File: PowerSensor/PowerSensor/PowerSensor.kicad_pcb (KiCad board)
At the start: 2 copper layers, 40.8 x 26.4 mm, 13 parts, among them J1 Screw_Terminal_01x02, J2 Screw_Terminal_01x05, J3 Screw_Terminal_01x02, J4 Screw_Terminal_01x02, U1 ACS712ELCTR-20A-T_NRND

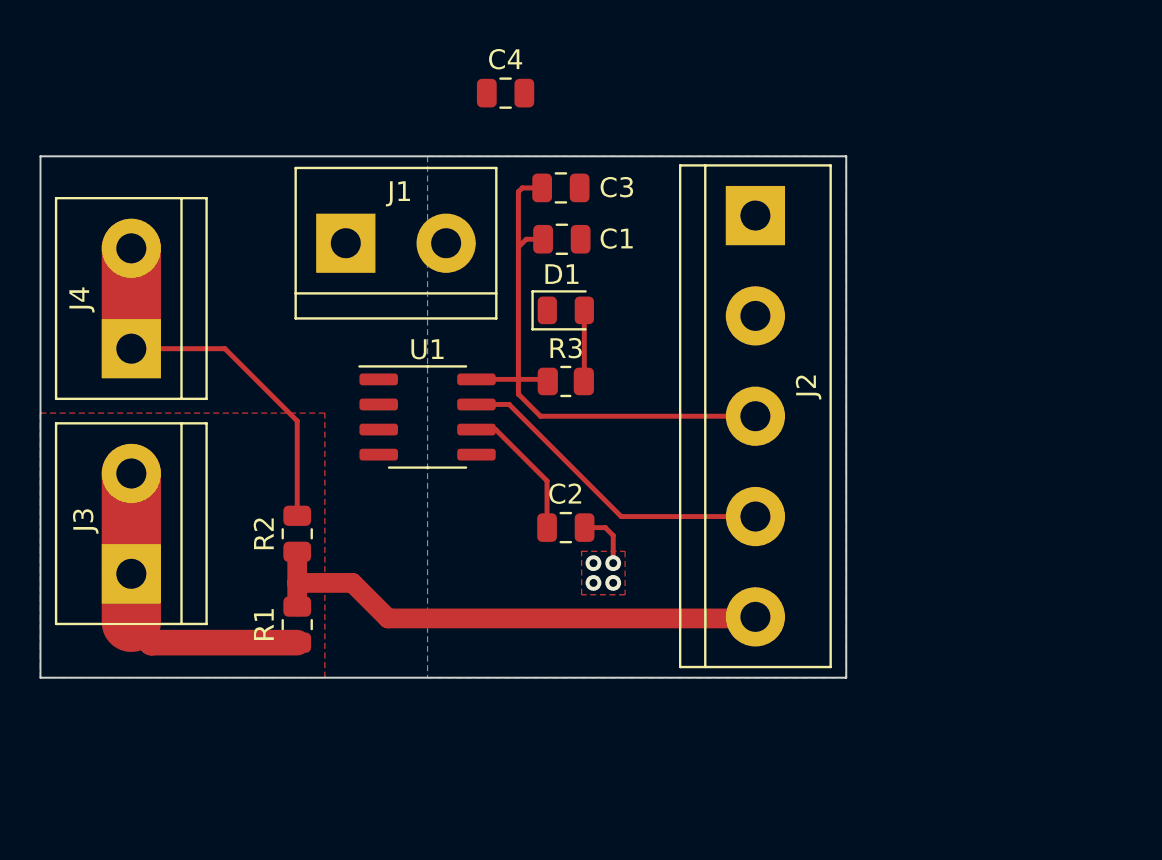
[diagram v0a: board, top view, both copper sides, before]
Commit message: Re desgin PCB
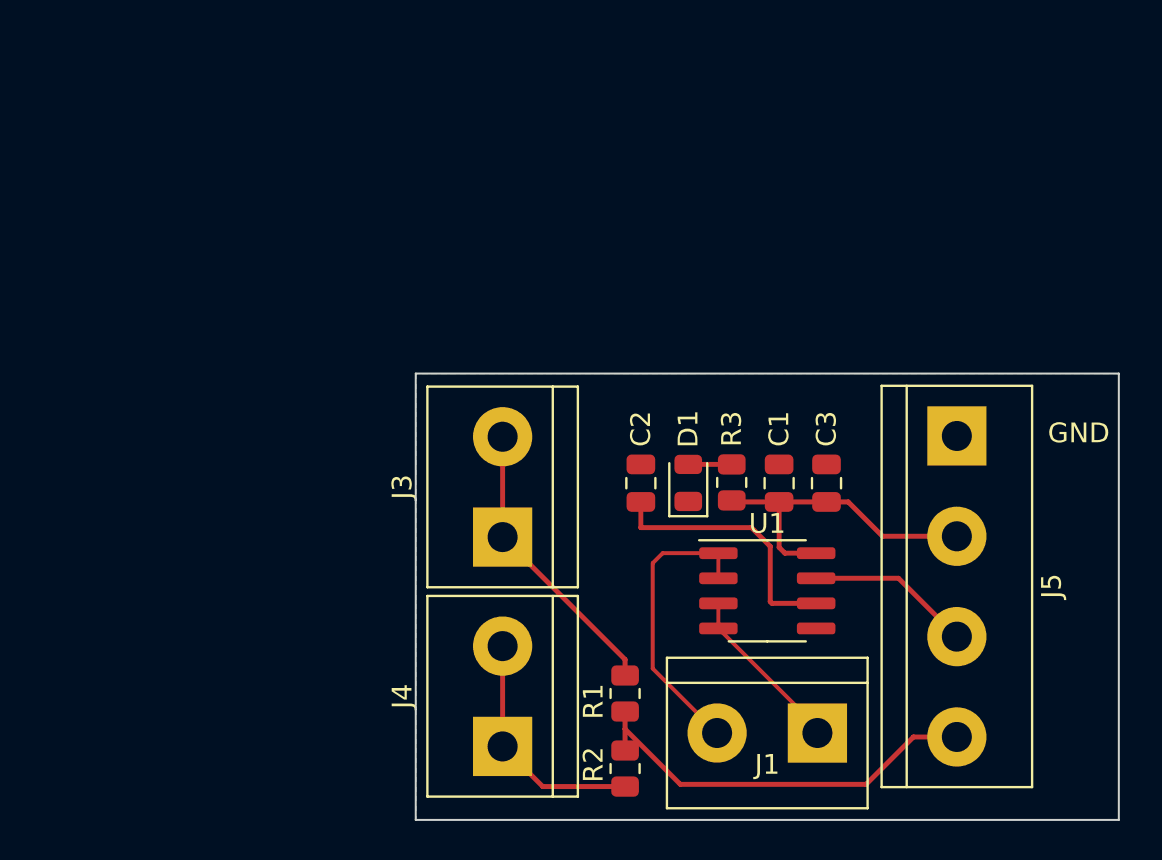
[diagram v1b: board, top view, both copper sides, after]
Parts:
- removed C4: 1uF, Capacitor_SMD:C_0805_2012Metric
- removed J2: Screw_Terminal_01x05, TerminalBlock:TerminalBlock_bornier-5_P5.08mm
- added J5: Screw_Terminal_01x04, TerminalBlock:TerminalBlock_bornier-4_P5.08mm, F.Cu at (118.8, 84.4)
- J1: value Screw_Terminal_01x02 -> Current Sens
- J3: value Screw_Terminal_01x02 -> BAT+
- J4: value Screw_Terminal_01x02 -> BAT-
- moved J1 34.4 mm to (111.7, 99.4), turned to 180 degrees
- moved J4 27.6 mm to (95.8, 100.1)
- moved R2 20.4 mm to (102.0, 101.2), turned to -90 degrees
- moved C3 20.1 mm to (112.2, 86.8), turned to 90 degrees
- moved U1 19.3 mm to (109.2, 92.2)
- moved J3 18.9 mm to (95.8, 89.5)
- moved R1 17.0 mm to (102.0, 97.4), turned to -90 degrees
- moved C1 16.5 mm to (109.8, 86.8), turned to 90 degrees
- moved D1 10.7 mm to (105.2, 86.7), turned to 90 degrees
- moved R3 9.83 mm to (107.4, 86.7), turned to 90 degrees
- moved C2 4.42 mm to (102.8, 86.8), turned to 90 degrees
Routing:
- net IN+: track 0.00 -> 14.8 mm
- net +5V: track 29.1 -> 16.4 mm
- net IN-: track 0.00 -> 8.64 mm
- net VIOUT: track 16.5 -> 8.35 mm
- net Battery(-): track 19.8 -> 12.1 mm
- net Net-(U1-FILTER): track 7.02 -> 13.4 mm
- net Vsens: track 26.8 -> 20.9 mm
- net GND: track 3.02 -> 0.00 mm, vias 4 -> 0
- net Battery(+): track 16.4 -> 14.7 mm
- net Net-(D1-A): track 3.61 -> 2.20 mm
- removed copper zone on F.Cu, net Battery(+)
- removed copper zone on F.Cu, net GND
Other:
- board size 40.8 x 26.4 mm -> 35.6 x 22.6 mm
- board text added: "+5V"
- board text added: "GND"
- board text added: "ISens"
- board text added: "VSens"
